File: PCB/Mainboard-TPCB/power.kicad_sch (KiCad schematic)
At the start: 4 parts, among them J15 Conn_01x02, U1 AMS1117-3.3

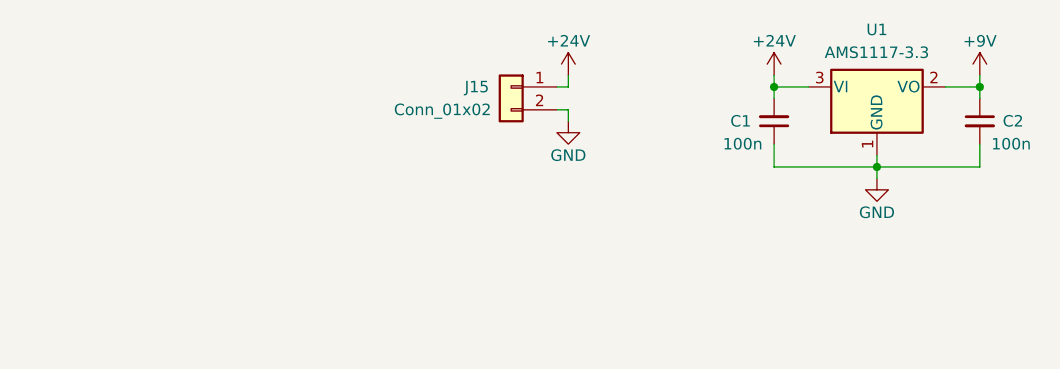
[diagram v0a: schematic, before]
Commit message: TPCB files V2
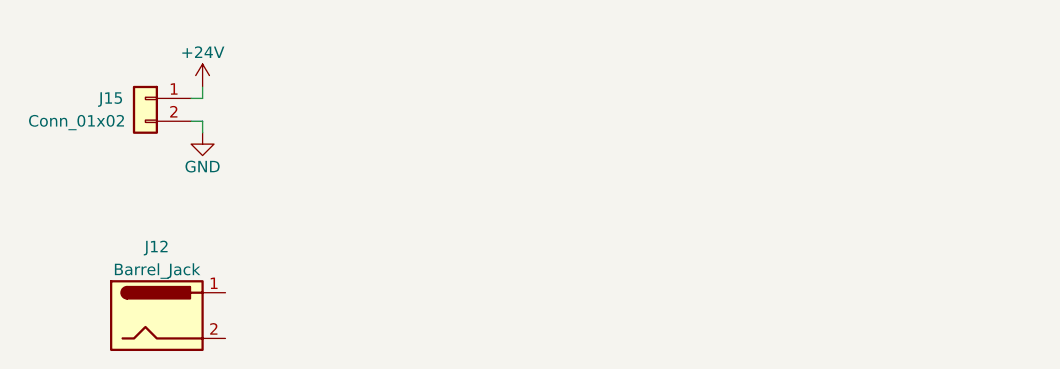
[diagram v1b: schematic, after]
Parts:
- removed C1, C2: 100n, Capacitor_SMD:C_0603_1608Metric, symbol Device:C_Small
- removed U1: AMS1117-3.3, Package_TO_SOT_SMD:SOT-223-3_TabPin2, symbol Regulator_Linear:AMS1117-3.3
- added J12: Barrel_Jack, Connector_BarrelJack:BarrelJack_GCT_DCJ200-10-A_Horizontal, symbol Connector:Barrel_Jack
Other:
- moved on the sheet: J15
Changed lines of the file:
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@@
     (company "ZOUDIO")
   )
-  (junction (at 158.75 96.52) (diameter 0) (color 0 0 0 0)
-  )
-  (junction (at 147.32 87.63) (diameter 0) (color 0 0 0 0)
-  )
-  (junction (at 170.18 87.63) (diameter 0) (color 0 0 0 0)
-  )
-  (wire (pts (xy 151.13 87.63) (xy 147.32 87.63))
+  (wire (pts (xy 82.55 88.9) (xy 83.82 88.9))
     (stroke (width 0) (type default) (color 0 0 0 0))
   )
-  (wire (pts (xy 147.32 86.36) (xy 147.32 87.63))
+  (wire (pts (xy 83.82 87.63) (xy 83.82 88.9))
     (stroke (width 0) (type default) (color 0 0 0 0))
   )
-  (wire (pts (xy 170.18 86.36) (xy 170.18 87.63))
+  (wire (pts (xy 83.82 91.44) (xy 83.82 92.71))
     (stroke (width 0) (type default) (color 0 0 0 0))
   )
-  (wire (pts (xy 147.32 96.52) (xy 158.75 96.52))
+  (wire (pts (xy 82.55 91.44) (xy 83.82 91.44))
     (stroke (width 0) (type default) (color 0 0 0 0))
   )
-  (wire (pts (xy 147.32 93.98) (xy 147.32 96.52))
-    (stroke (width 0) (type default) (color 0 0 0 0))
-  )
-  (wire (pts (xy 123.19 87.63) (xy 124.46 87.63))
-    (stroke (width 0) (type default) (color 0 0 0 0))
-  )
-  (wire (pts (xy 124.46 86.36) (xy 124.46 87.63))
-    (stroke (width 0) (type default) (color 0 0 0 0))
-  )
-  (wire (pts (xy 158.75 95.25) (xy 158.75 96.52))
-    (stroke (width 0) (type default) (color 0 0 0 0))
-  )
-  (wire (pts (xy 170.18 93.98) (xy 170.18 96.52))
-    (stroke (width 0) (type default) (color 0 0 0 0))
-  )
-  (wire (pts (xy 124.46 90.17) (xy 124.46 91.44))
-    (stroke (width 0) (type default) (color 0 0 0 0))
-  )
-  (wire (pts (xy 158.75 96.52) (xy 158.75 97.79))
-    (stroke (width 0) (type default) (color 0 0 0 0))
-  )
-  (wire (pts (xy 123.19 90.17) (xy 124.46 90.17))
-    (stroke (width 0) (type default) (color 0 0 0 0))
-  )
-  (wire (pts (xy 158.75 96.52) (xy 170.18 96.52))
-    (stroke (width 0) (type default) (color 0 0 0 0))
-  )
-  (wire (pts (xy 170.18 87.63) (xy 170.18 88.9))
-    (stroke (width 0) (type default) (color 0 0 0 0))
-  )
-  (wire (pts (xy 147.32 87.63) (xy 147.32 88.9))
-    (stroke (width 0) (type default) (color 0 0 0 0))
-  )
-  (wire (pts (xy 166.37 87.63) (xy 170.18 87.63))
-    (stroke (width 0) (type default) (color 0 0 0 0))
-  )
-  (symbol (lib_id "power:+24V") (at 147.32 86.36 0) (unit 1)
+  (symbol (lib_id "power:GND") (at 83.82 92.71 0) (unit 1)
     (in_bom yes) (on_board yes)
-    (property "Reference" "#PWR0110" (id 0) (at 147.32 90.17 0)
+    (property "Reference" "#PWR0116" (id 0) (at 83.82 99.06 0)
       (effects (font (size 1.27 1.27)) hide)
     )
-    (property "Value" "+24V" (id 1) (at 147.32 82.55 0))
-    (property "Footprint" "" (id 2) (at 147.32 86.36 0)
+    (property "Value" "GND" (id 1) (at 83.82 96.52 0))
+    (property "Footprint" "" (id 2) (at 83.82 92.71 0)
       (effects (font (size 1.27 1.27)) hide)
     )
-    (property "Datasheet" "" (id 3) (at 147.32 86.36 0)
+    (property "Datasheet" "" (id 3) (at 83.82 92.71 0)
       (effects (font (size 1.27 1.27)) hide)
     )
     (pin "1")
   )
-  (symbol (lib_id "power:+9V") (at 170.18 86.36 0) (unit 1)
-    (in_bom yes) (on_board yes)
-    (property "Reference" "#PWR0118" (id 0) (at 170.18 90.17 0)
+  (symbol (lib_id "Connector:Barrel_Jack") (at 78.74 113.03 0) (unit 1)
+    (in_bom yes) (on_board yes) (fields_autoplaced)
+    (property "Reference" "J12" (id 0) (at 78.74 105.41 0))
+    (property "Value" "Barrel_Jack" (id 1) (at 78.74 107.95 0))
+    (property "Footprint" "Connector_BarrelJack:BarrelJack_GCT_DCJ200-10-A_Horizontal" (id 2) (at 80.01 114.046 0)
       (effects (font (size 1.27 1.27)) hide)
     )
-    (property "Value" "+9V" (id 1) (at 170.18 82.55 0))
-    (property "Footprint" "" (id 2) (at 170.18 86.36 0)
-      (effects (font (size 1.27 1.27)) hide)
-    )
-    (property "Datasheet" "" (id 3) (at 170.18 86.36 0)
-      (effects (font (size 1.27 1.27)) hide)
-    )
-    (pin "1")
-  )
-  (symbol (lib_id "power:GND") (at 124.46 91.44 0) (unit 1)
-    (in_bom yes) (on_board yes)
-    (property "Reference" "#PWR0116" (id 0) (at 124.46 97.79 0)
-      (effects (font (size 1.27 1.27)) hide)
-    )
-    (property "Value" "GND" (id 1) (at 124.46 95.25 0))
-    (property "Footprint" "" (id 2) (at 124.46 91.44 0)
-      (effects (font (size 1.27 1.27)) hide)
-    )
-    (property "Datasheet" "" (id 3) (at 124.46 91.44 0)
-      (effects (font (size 1.27 1.27)) hide)
-    )
-    (pin "1")
-  )
-  (symbol (lib_id "power:GND") (at 158.75 97.79 0) (unit 1)
-    (in_bom yes) (on_board yes)
-    (property "Reference" "#PWR0114" (id 0) (at 158.75 104.14 0)
-      (effects (font (size 1.27 1.27)) hide)
-    )
-    (property "Value" "GND" (id 1) (at 158.75 101.6 0))
-    (property "Footprint" "" (id 2) (at 158.75 97.79 0)
-      (effects (font (size 1.27 1.27)) hide)
-    )
-    (property "Datasheet" "" (id 3) (at 158.75 97.79 0)
-      (effects (font (size 1.27 1.27)) hide)
-    )
-    (pin "1")
-  )
-  (symbol (lib_id "power:+24V") (at 124.46 86.36 0) (unit 1)
-    (in_bom yes) (on_board yes)
-    (property "Reference" "#PWR0117" (id 0) (at 124.46 90.17 0)
-      (effects (font (size 1.27 1.27)) hide)
-    )
-    (property "Value" "+24V" (id 1) (at 124.46 82.55 0))
-    (property "Footprint" "" (id 2) (at 124.46 86.36 0)
-      (effects (font (size 1.27 1.27)) hide)
-    )
-    (property "Datasheet" "" (id 3) (at 124.46 86.36 0)
-      (effects (font (size 1.27 1.27)) hide)
-    )
-    (pin "1")
-  )
-  (symbol (lib_id "Device:C_Small") (at 147.32 91.44 0) (mirror x) (unit 1)
-    (in_bom yes) (on_board yes)
-    (property "Reference" "C1" (id 0) (at 144.78 91.44 0)
-      (effects (font (size 1.27 1.27)) (justify right))
-    )
-    (property "Value" "100n" (id 1) (at 146.05 93.98 0)
-      (effects (font (size 1.27 1.27)) (justify right))
-    )
-    (property "Footprint" "Capacitor_SMD:C_0603_1608Metric" (id 2) (at 147.32 91.44 0)
-      (effects (font (size 1.27 1.27)) hide)
-    )
-    (property "Datasheet" "~" (id 3) (at 147.32 91.44 0)
+    (property "Datasheet" "~" (id 3) (at 80.01 114.046 0)
       (effects (font (size 1.27 1.27)) hide)
     )
@@
     (pin "2")
   )
-  (symbol (lib_id "Regulator_Linear:AMS1117-3.3") (at 158.75 87.63 0) (unit 1)
+  (symbol (lib_id "power:+24V") (at 83.82 87.63 0) (unit 1)
     (in_bom yes) (on_board yes)
-    (property "Reference" "U1" (id 0) (at 158.75 81.28 0))
-    (property "Value" "AMS1117-3.3" (id 1) (at 158.75 83.82 0))
-    (property "Footprint" "Package_TO_SOT_SMD:SOT-223-3_TabPin2" (id 2) (at 158.75 82.55 0)
+    (property "Reference" "#PWR0117" (id 0) (at 83.82 91.44 0)
       (effects (font (size 1.27 1.27)) hide)
     )
-    (property "Datasheet" "http://www.advanced-monolithic.com/pdf/ds1117.pdf" (id 3) (at 161.29 93.98 0)
+    (property "Value" "+24V" (id 1) (at 83.82 83.82 0))
+    (property "Footprint" "" (id 2) (at 83.82 87.63 0)
+      (effects (font (size 1.27 1.27)) hide)
+    )
+    (property "Datasheet" "" (id 3) (at 83.82 87.63 0)
       (effects (font (size 1.27 1.27)) hide)
     )
     (pin "1")
-    (pin "2")
-    (pin "3")
   )
-  (symbol (lib_id "Device:C_Small") (at 170.18 91.44 0) (unit 1)
+  (symbol (lib_id "Connector_Generic:Conn_01x02") (at 77.47 88.9 0) (mirror y) (unit 1)
     (in_bom yes) (on_board yes)
-    (property "Reference" "C2" (id 0) (at 172.72 91.44 0)
-      (effects (font (size 1.27 1.27)) (justify left))
-    )
-    (property "Value" "100n" (id 1) (at 171.45 93.98 0)
-      (effects (font (size 1.27 1.27)) (justify left))
-    )
-    (property "Footprint" "Capacitor_SMD:C_0603_1608Metric" (id 2) (at 170.18 91.44 0)
+    (property "Reference" "J15" (id 0) (at 73.66 88.9 0))
+    (property "Value" "Conn_01x02" (id 1) (at 69.85 91.44 0))
+    (property "Footprint" "Connector_Phoenix_MSTB:PhoenixContact_MSTBA_2,5_2-G-5,08_1x02_P5.08mm_Horizontal" (id 2) (at 77.47 88.9 0)
       (effects (font (size 1.27 1.27)) hide)
     )
-    (property "Datasheet" "~" (id 3) (at 170.18 91.44 0)
+    (property "Datasheet" "~" (id 3) (at 77.47 88.9 0)
       (effects (font (size 1.27 1.27)) hide)
     )
-    (pin "1")
-    (pin "2")
-  )
-  (symbol (lib_id "Connector_Generic:Conn_01x02") (at 118.11 87.63 0) (mirror y) (unit 1)
-    (in_bom yes) (on_board yes)
-    (property "Reference" "J15" (id 0) (at 114.3 87.63 0))
-    (property "Value" "Conn_01x02" (id 1) (at 110.49 90.17 0))
-    (property "Footprint" "Connector_Phoenix_MSTB:PhoenixContact_MSTBA_2,5_2-G-5,08_1x02_P5.08mm_Horizontal" (id 2) (at 118.11 87.63 0)
-      (effects (font (size 1.27 1.27)) hide)
-    )
-    (property "Datasheet" "~" (id 3) (at 118.11 87.63 0)
-      (effects (font (size 1.27 1.27)) hide)
-    )
